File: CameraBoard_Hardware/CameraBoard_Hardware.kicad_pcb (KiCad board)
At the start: 2 copper layers, 61 x 100 mm, 41 parts, among them J1 BNC_75_OHM_HORIZ, J2 BNC_75_OHM_HORIZ, U1 TM4C129E_Launchpad, U2 AP1059, U3 MAX4314ESD+, U4 MAX4314ESD+

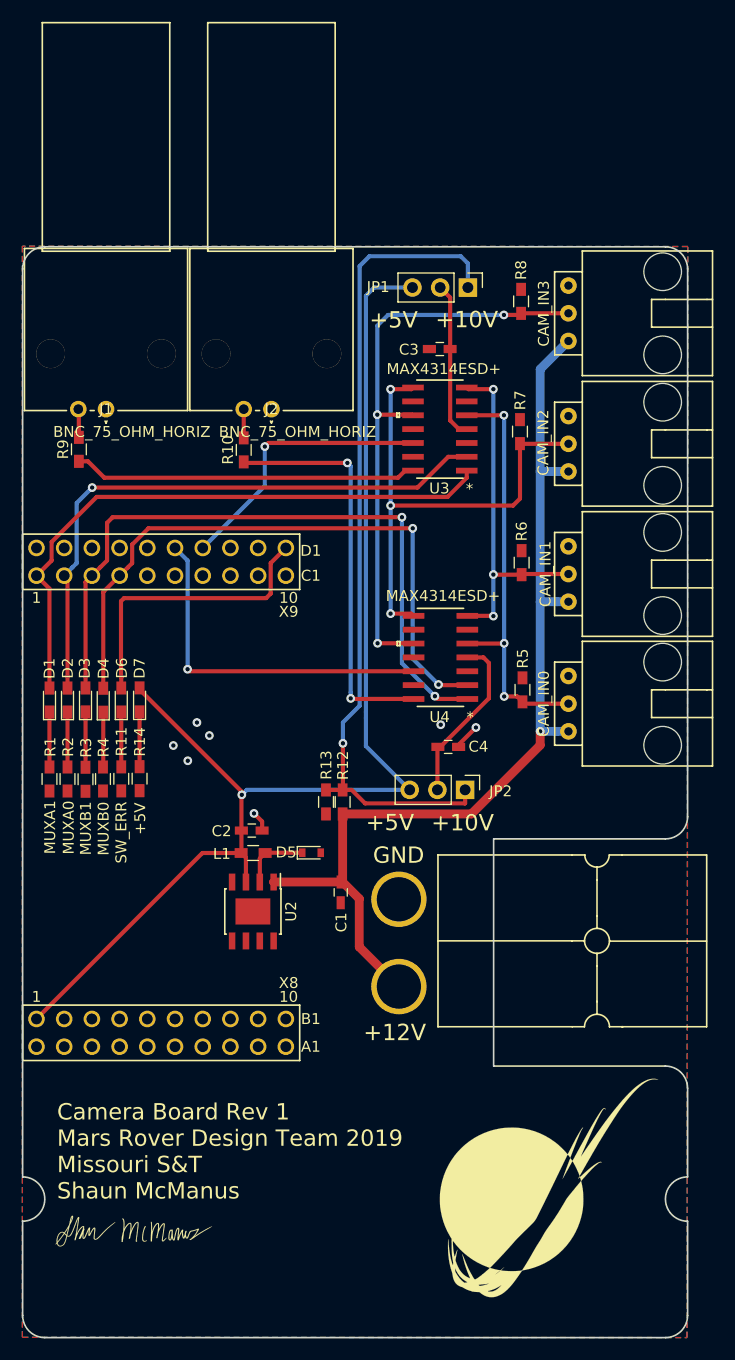
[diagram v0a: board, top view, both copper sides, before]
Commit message: Re-Routed Traces
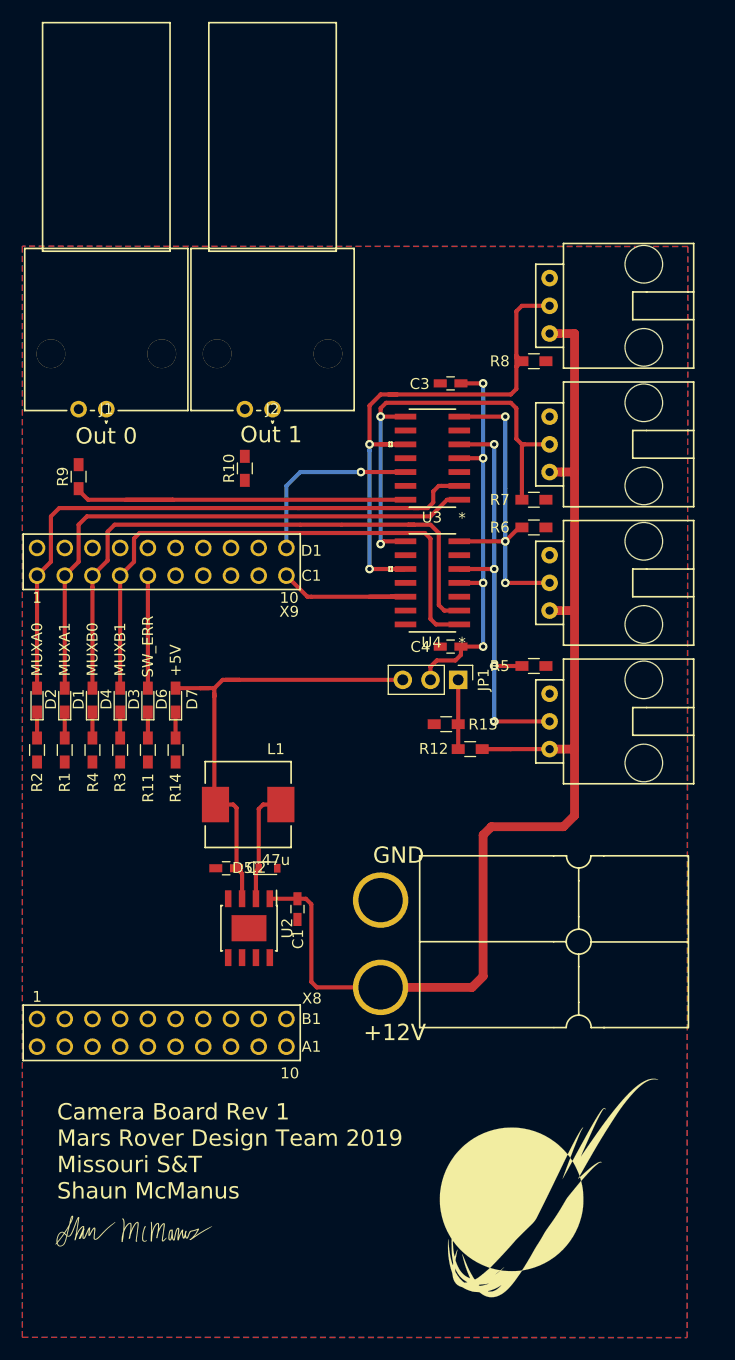
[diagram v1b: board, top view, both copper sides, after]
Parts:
- removed CAM_IN0: CAM_0, MRDT_Connectors:MOLEX_SL_03_Horizontal
- removed CAM_IN1: CAM_1, MRDT_Connectors:MOLEX_SL_03_Horizontal
- removed CAM_IN2: CAM_2, MRDT_Connectors:MOLEX_SL_03_Horizontal
- removed CAM_IN3: CAM_3, MRDT_Connectors:MOLEX_SL_03_Horizontal
- removed JP2: Jumper_NC_Dual, Pin_Headers:Pin_Header_Straight_1x03_Pitch2.54mm
- added Conn3: CAM_0, MRDT_Connectors:MOLEX_SL_03_Horizontal, F.Cu at (134.6, 99.1)
- added Conn4: CAM_1, MRDT_Connectors:MOLEX_SL_03_Horizontal, F.Cu at (134.6, 86.4)
- added Conn5: CAM_2, MRDT_Connectors:MOLEX_SL_03_Horizontal, F.Cu at (134.6, 73.7)
- added Conn6: CAM_3, MRDT_Connectors:MOLEX_SL_03_Horizontal, F.Cu at (134.6, 61.0)
- L1: footprint Inductors_SMD:L_0603_HandSoldering -> MRDT_Passives:DR74_330_R
- moved JP1 36.0 mm to (126.2, 95.2)
- moved R13 13.1 mm to (125.1, 99.3), turned to 180 degrees
- moved R12 12.7 mm to (127.3, 101.6), turned to 180 degrees
- moved C4 9.20 mm to (125.5, 92.2), turned to 180 degrees
- moved U4 6.87 mm to (123.9, 86.4)
- moved R7 6.38 mm to (133.2, 78.7), turned to 180 degrees
- moved R8 5.61 mm to (133.2, 66.0), turned to 180 degrees
- moved L1 4.47 mm to (107.0, 106.7)
- moved C1 4.25 mm to (111.5, 116.3)
- moved D5 4.23 mm to (108.8, 112.5)
- moved R14 4.22 mm to (100.3, 101.7)
- moved C2 4.18 mm to (105.0, 112.5), turned to 0 degrees
- moved R3 4.16 mm to (95.2, 101.7)
- moved R2 3.85 mm to (87.6, 101.7)
- moved R11 3.59 mm to (97.8, 101.7)
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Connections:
- C3 pad 1: Net-(C3-Pad1) -> /MUX_PWR
- C4 pad 1: Net-(C4-Pad1) -> /MUX_PWR
- JP1 pad 2: Net-(C3-Pad1) -> /MUX_PWR
- U1 pad +3V3: Net-(U1-Pad+3V3) -> (no net)
- U1 pad PA6: Net-(U1-PadPA6) -> (no net)
- U1 pad PB2: Net-(U1-PadPB2) -> (no net)
- U1 pad PB3: Net-(U1-PadPB3) -> (no net)
- U1 pad PC4: Net-(U1-PadPC4) -> (no net)
- U1 pad PC5: Net-(U1-PadPC5) -> (no net)
- U1 pad PC6: Net-(U1-PadPC6) -> (no net)
- U1 pad PC7: Net-(U1-PadPC7) -> (no net)
- U1 pad PD0: MUXA_SHDN -> (no net)
- U1 pad PD1: MUXB_SHDN -> (no net)
- U1 pad PD3: Net-(U1-PadPD3) -> (no net)
- U1 pad PD7: Net-(U1-PadPD7) -> (no net)
- U1 pad PE0: Net-(U1-PadPE0) -> (no net)
- U1 pad PE1: Net-(U1-PadPE1) -> (no net)
- U1 pad PE2: Net-(U1-PadPE2) -> (no net)
- U1 pad PE3: Net-(U1-PadPE3) -> (no net)
- U1 pad PE4: Net-(U1-PadPE4) -> (no net)
- U1 pad PE5: Net-(U1-PadPE5) -> (no net)
- U1 pad PF1: MUXA1 -> MUXA0
- U1 pad PF2: MUXA0 -> MUXA1
- U1 pad PF3: MUXB1 -> MUXB0
- U1 pad PG0: MUXB0 -> MUXB1
- U1 pad PH2: Net-(U1-PadPH2) -> (no net)
- U1 pad PH3: Net-(U1-PadPH3) -> (no net)
- U1 pad PL0: Net-(U1-PadPL0) -> (no net)
- U1 pad PL1: Net-(U1-PadPL1) -> (no net)
- U1 pad PL2: Net-(U1-PadPL2) -> (no net)
- U1 pad PL3: Net-(U1-PadPL3) -> MUXB_SHDN
- U1 pad PL4: Net-(U1-PadPL4) -> SW_ERR
- U1 pad PL5: Net-(U1-PadPL5) -> (no net)
- U1 pad PM3: Net-(U1-PadPM3) -> (no net)
- U1 pad PM4: Net-(U1-PadPM4) -> (no net)
- U1 pad PM5: Net-(U1-PadPM5) -> (no net)
- U1 pad PN2: Net-(U1-PadPN2) -> (no net)
- U1 pad PN3: Net-(U1-PadPN3) -> (no net)
- U1 pad PP2: SW_ERR -> MUXA_SHDN
- U1 pad Rese: Net-(U1-PadRese) -> (no net)
- U3 pad 3: Net-(U3-Pad3) -> (no net)
- U3 pad 4: Net-(C3-Pad1) -> /MUX_PWR
- U3 pad 6: Net-(U3-Pad6) -> (no net)
- U3 pad 9: Net-(U3-Pad9) -> (no net)
- U4 pad 3: Net-(U4-Pad3) -> (no net)
- U4 pad 4: Net-(C4-Pad1) -> /MUX_PWR
- U4 pad 6: Net-(U4-Pad6) -> (no net)
- U4 pad 9: Net-(U4-Pad9) -> (no net)
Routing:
- net +10V: track 75.9 -> 6.35 mm, vias 1 -> 0
- net +5V: track 114.1 -> 44.7 mm, vias 1 -> 0
- net /MUX_PWR: track 0.00 -> 40.8 mm, vias 0 -> 4
- net CAM_OUT1: track 37.4 -> 0.00 mm, vias 2 -> 0
- net +12V: track 92.3 -> 111.3 mm, vias 1 -> 0
- net SW_ERR: track 26.7 -> 10.3 mm
- net MUXB_SHDN: track 32.4 -> 16.4 mm, vias 1 -> 0
- net Net-(C4-Pad1): track 15.9 -> 0.00 mm
- net Net-(C3-Pad1): track 14.4 -> 0.00 mm
- net MUXB1: track 63.9 -> 52.1 mm, vias 2 -> 0
- net CAM_IN0: track 38.8 -> 48.6 mm, vias 3 -> 4
- net MUXA_SHDN: track 25.4 -> 17.2 mm
- net CAM_IN2: track 46.5 -> 41.1 mm, vias 3 -> 2
- net GND: track 4.32 -> 0.00 mm, vias 7 -> 0
- net Net-(D5-Pad1): track 6.27 -> 10.5 mm
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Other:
- board outline removed
- board text added: "Out 0"
- board text added: "Out 1"
- board text removed: "+10V"
